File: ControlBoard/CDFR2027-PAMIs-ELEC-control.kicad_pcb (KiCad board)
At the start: 4 copper layers, 109.8 x 79.8 mm, 92 parts, among them J1 Conn_01x04_Pin, Q1 PMOS, U1 USBLC6-2P6

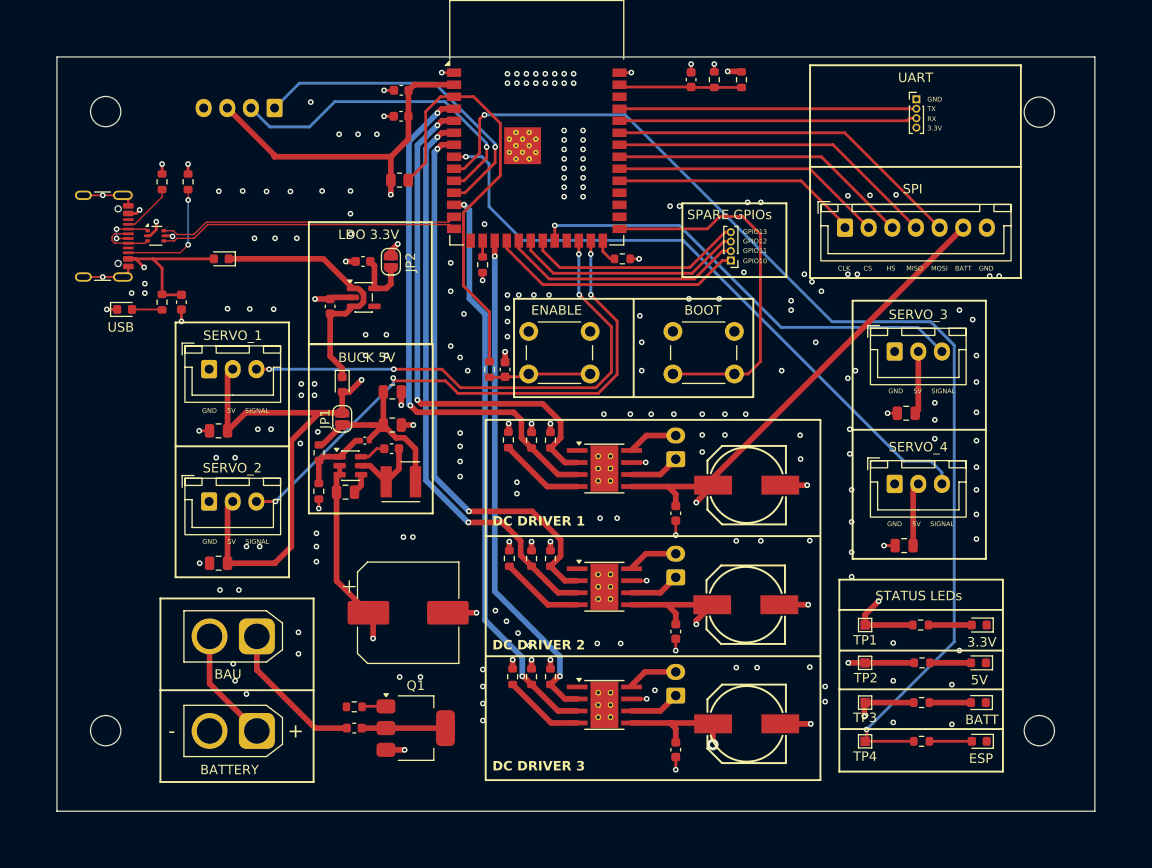
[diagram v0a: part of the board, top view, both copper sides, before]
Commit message: (cleanup): gain space
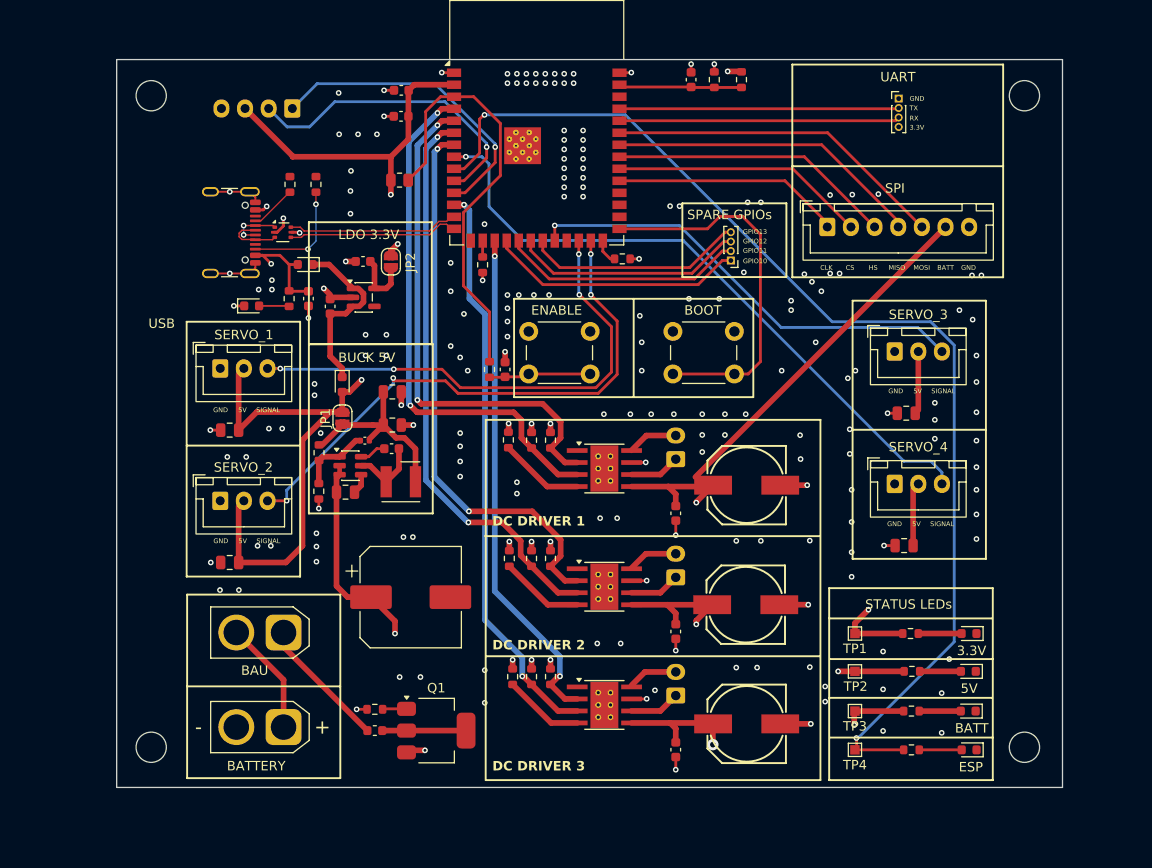
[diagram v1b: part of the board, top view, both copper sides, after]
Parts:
- moved R21 13.5 mm to (100.0, 75.7)
- moved R22 13.5 mm to (102.8, 75.7)
- moved C18 13.4 mm to (102.0, 87.8)
- moved USB_C1 13.4 mm to (92.7, 80.8)
- moved R20 13.4 mm to (99.9, 87.8)
- moved U1 13.4 mm to (99.2, 80.8)
- moved USB1 13.4 mm to (95.9, 88.5)
- moved D2 8.90 mm to (101.6, 84.2)
- moved H3 5.12 mm to (85.3, 135.2)
- moved H1 5.10 mm to (85.3, 66.3)
- moved REF** 3.09 mm to (163.2, 128.8)
- moved BAU1 2.85 mm to (99.3, 123.1)
- moved C_BATT1 2.85 mm to (99.3, 133.1)
- moved H4 2.36 mm to (177.7, 135.2)
- moved H2 2.34 mm to (177.7, 66.3)
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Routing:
- net /External IO/USB_D-: track 31.6 -> 18.0 mm
- net /External IO/USB_D+: track 31.6 -> 18.0 mm
- net Net-(D1-K): track 27.9 -> 18.8 mm
- net BATT: track 304.9 -> 311.1 mm
- net USB: track 30.0 -> 24.5 mm
- net GND: track 70.9 -> 66.7 mm, vias 230 -> 204
- net /External IO/Handshake: track 32.0 -> 30.0 mm
- net /External IO/MOSI: track 38.0 -> 36.1 mm
- net /External IO/CS: track 28.9 -> 27.0 mm
- net /External IO/SDA: track 34.6 -> 32.7 mm
- net /External IO/SCL: track 34.7 -> 32.8 mm
- net /External IO/CLK: track 26.1 -> 24.2 mm
- net /External IO/TXD0: track 31.4 -> 29.6 mm
- net Net-(BAU1-Pin_1): track 15.6 -> 14.0 mm
- net /External IO/MISO: track 35.0 -> 33.4 mm
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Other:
- board size 109.8 x 79.8 mm -> 100 x 77 mm
